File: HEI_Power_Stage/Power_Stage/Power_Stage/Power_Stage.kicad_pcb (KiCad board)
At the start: 2 copper layers, 1 part, among them Q1 EPC2304ENGRT

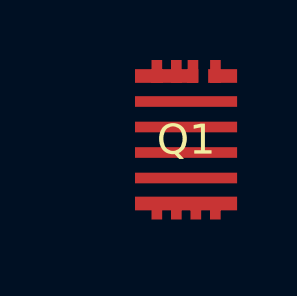
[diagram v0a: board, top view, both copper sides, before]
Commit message: second try for kicad libs
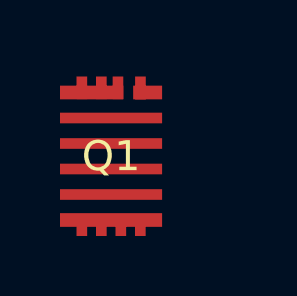
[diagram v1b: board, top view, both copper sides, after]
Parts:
- moved Q1 2.56 mm to (130.8, 83.4)
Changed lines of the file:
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@@
   (net 7 "unconnected-(Q1-Pad7)")
   (footprint "GTSR_KiCAD_Footprints_SD:EPC2304_ECC" (layer "F.Cu")
-    (at 133.298994 82.808311)
+    (at 130.798994 83.358311)
     (tags "EPC2304ENGRT ")
     (property "Sheetfile" "Power_Stage.kicad_sch")
